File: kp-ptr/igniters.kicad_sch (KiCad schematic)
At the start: 48 parts, among them J10 Conn_01x02, J11 Conn_01x02, J12 Conn_01x02, J13 Conn_01x02, Q10 PMOS_SOT23, Q11 PMOS_SOT23, Q12 PMOS_SOT23, Q13 PMOS_SOT23, Q6 NMOS_SOT23, Q7 NMOS_SOT23, Q8 NMOS_SOT23, Q9 NMOS_SOT23

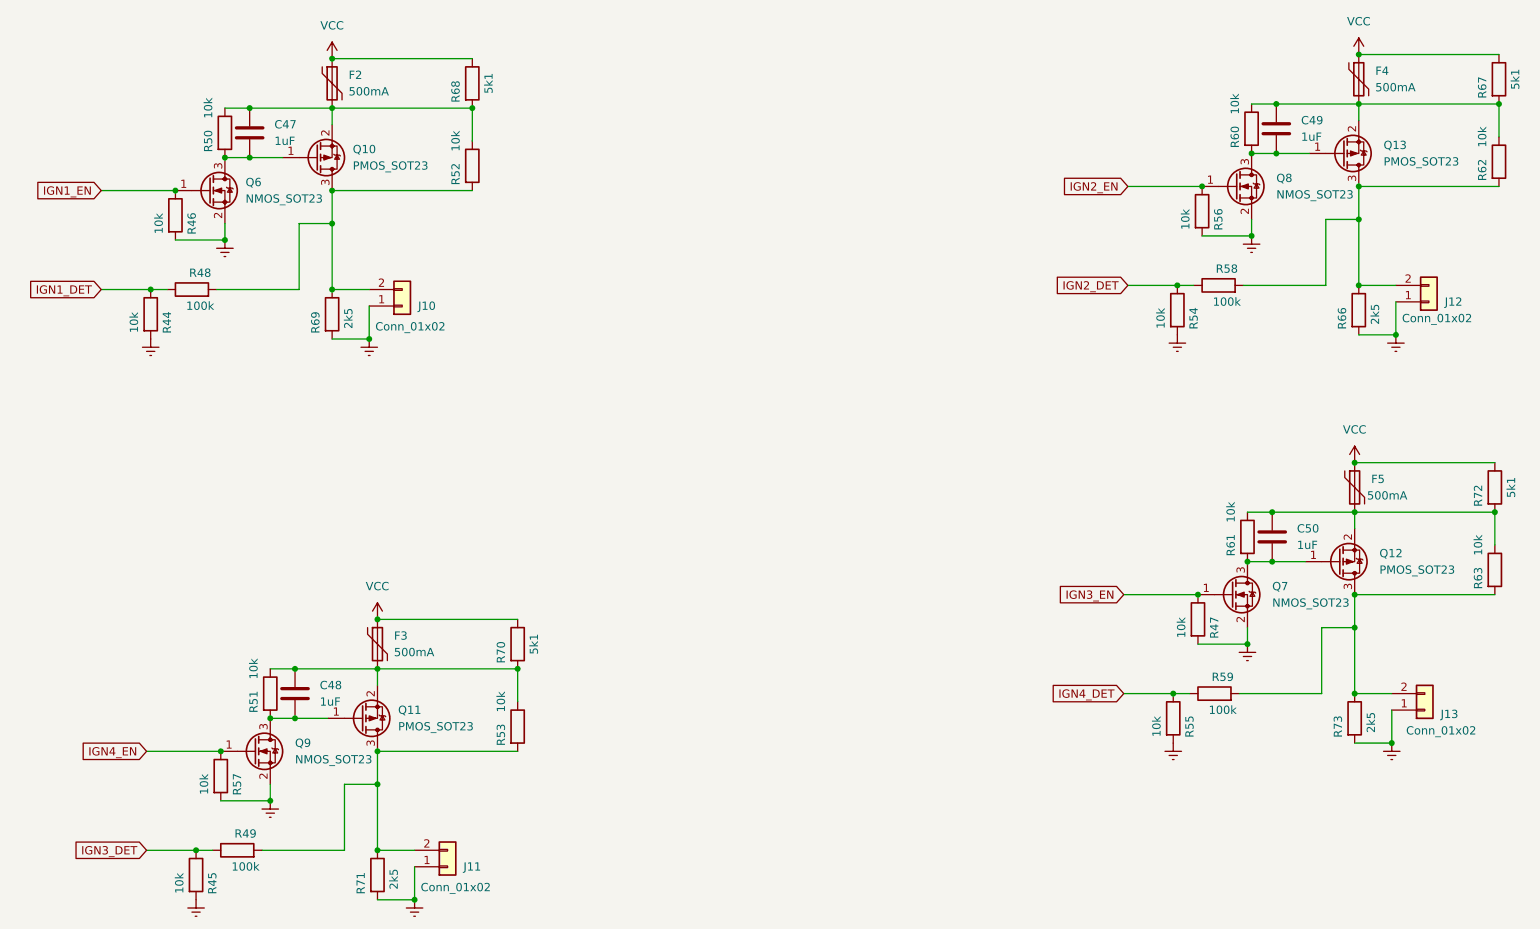
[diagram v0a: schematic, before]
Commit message: Igniters rework v2
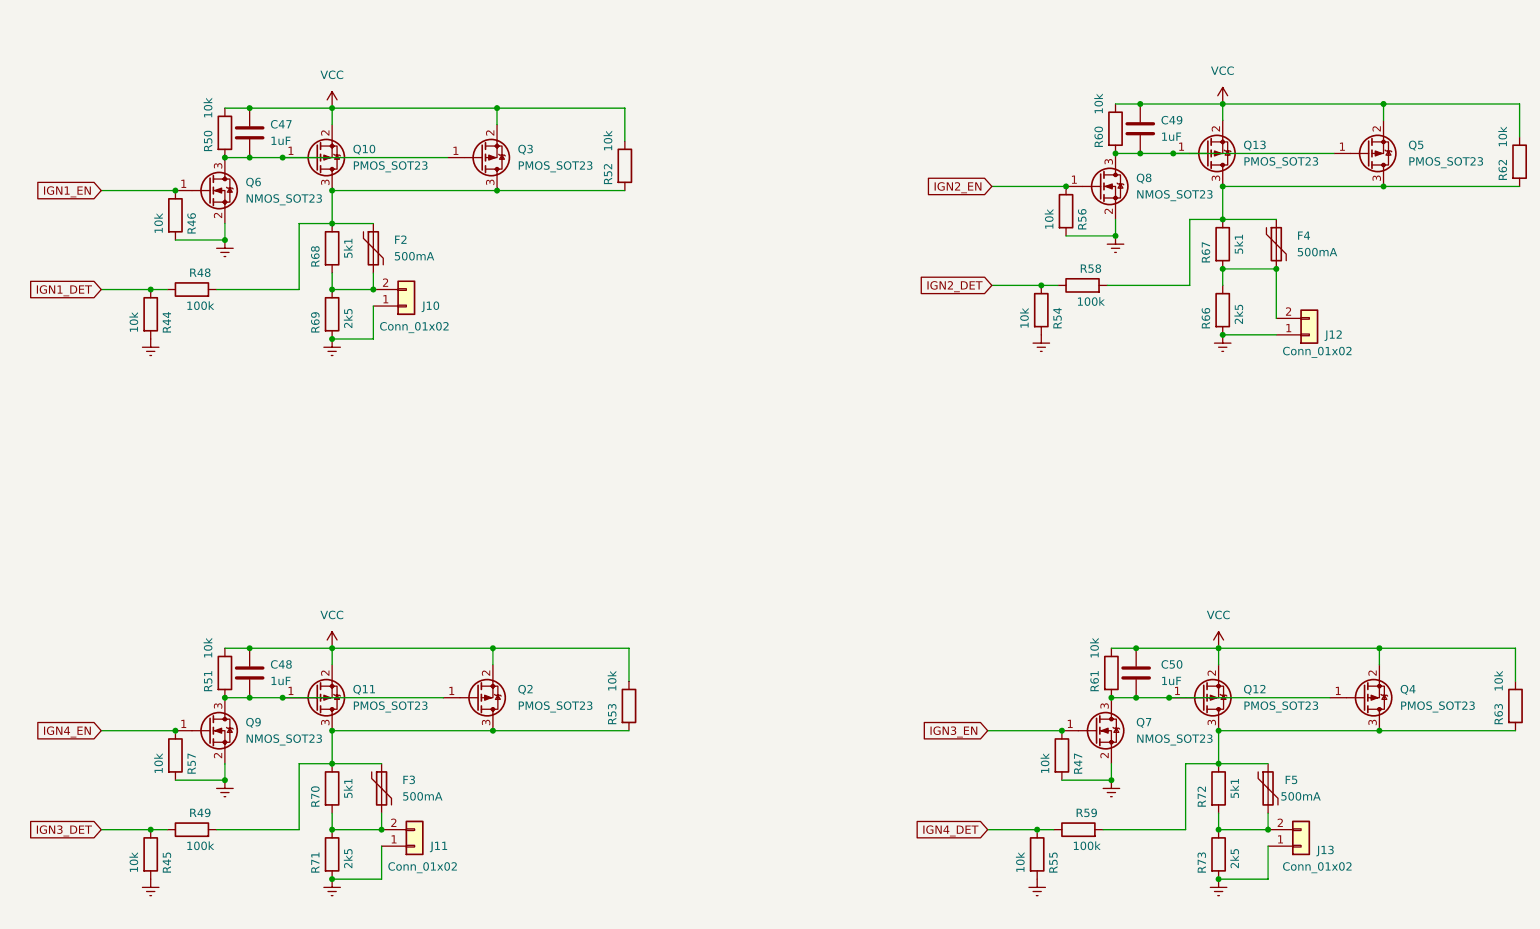
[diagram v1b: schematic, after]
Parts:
- added Q2, Q3, Q4, Q5: PMOS_SOT23, KP-PTR_lib:SOT-23, symbol Transistor_FET:IRLML6401
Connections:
- net VCC: now also C47.1, C48.1, C49.1, C50.1, Q10.2 (S), Q11.2 (S), Q12.2 (S), Q13.2 (S), R50.1, R51.1, R52.1, R53.1, R60.1, R61.1, R62.1, R63.1, Q2.2 (S), Q3.2 (S), Q4.2 (S), Q5.2 (S); no longer F2.1, F3.1, F4.1, F5.1, R67.1, R68.1, R70.1, R72.1
- net at C50.2, Q12.1 (G), Q7.3 (D)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: now also Q4.1 (G)
- net at Q12.3 (D), R59.2, R63.2: now also F5.1, R72.1, Q4.3 (D); no longer J13.2 (Pin_2), R73.1
- net at Q11.3 (D), R49.2, R53.2: now also F3.1, R70.1, Q2.3 (D); no longer J11.2 (Pin_2), R71.1
- net at Q10.3 (D), R48.2, R52.2: now also F2.1, R68.1, Q3.3 (D); no longer J10.2 (Pin_2), R69.1
- net at C49.2, Q13.1 (G), Q8.3 (D)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: now also Q5.1 (G)
- net at Q13.3 (D), R58.2, R62.2: now also F4.1, R67.1, Q5.3 (D); no longer J12.2 (Pin_2), R66.1
- net at C47.2, Q10.1 (G), Q6.3 (D)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: now also Q3.1 (G)
- net at C48.2, Q11.1 (G), Q9.3 (D)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: now also Q2.1 (G)
- new net: F5.2, J13.2 (Pin_2), R72.2, R73.1
- new net: F3.2, J11.2 (Pin_2), R70.2, R71.1
- new net: F2.2, J10.2 (Pin_2), R68.2, R69.1
- new net: F4.2, J12.2 (Pin_2), R66.1, R67.2
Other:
- moved on the sheet: C48, C49, C50, F2, F3, F4, F5, J10, J11, J12, J13, Q11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
